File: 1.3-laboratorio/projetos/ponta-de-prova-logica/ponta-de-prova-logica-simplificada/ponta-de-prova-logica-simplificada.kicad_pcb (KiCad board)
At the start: 2 copper layers, 36.8 x 63.5 mm, 21 parts, among them J1 Conn_01x02, J2 PONTA DE PROVA, U1 LM339

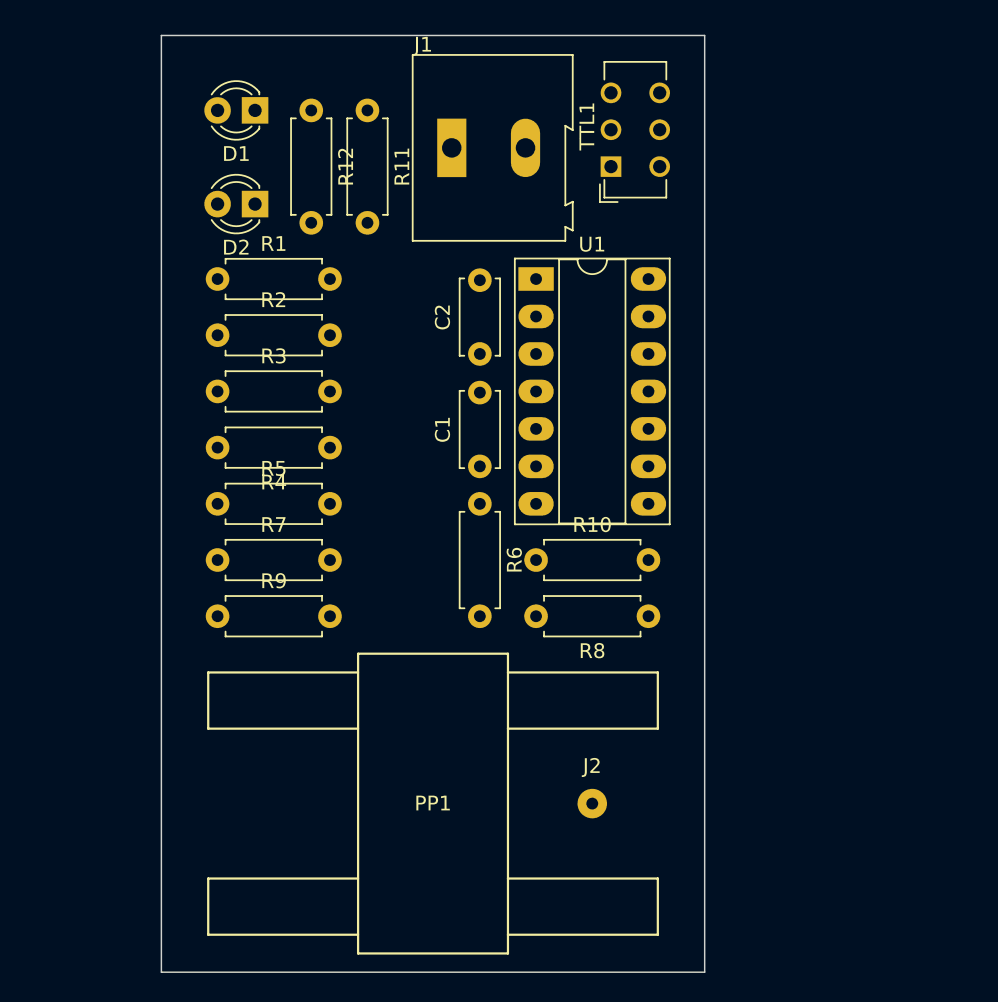
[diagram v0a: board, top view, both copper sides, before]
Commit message: Leiaute da PCB em andamento.
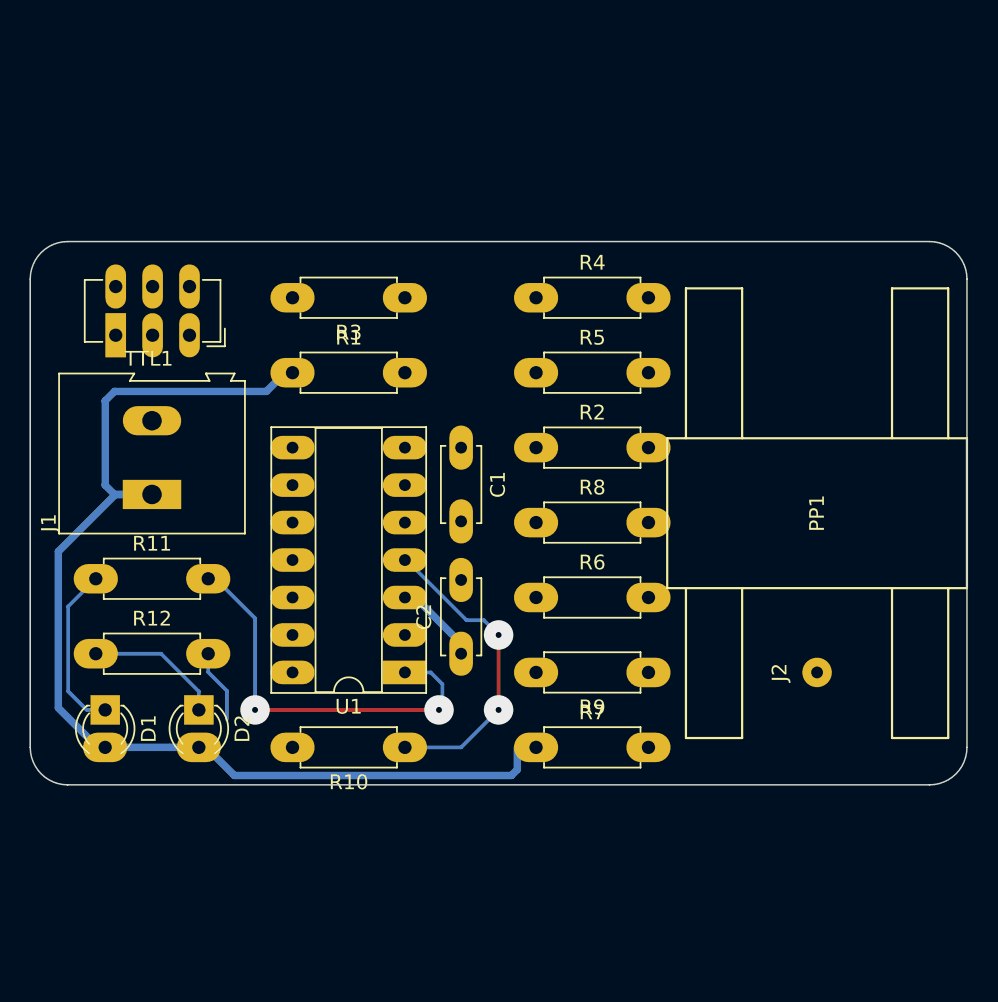
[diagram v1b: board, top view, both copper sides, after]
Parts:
- moved D1 41.9 mm to (134.6, 114.3), turned to 270 degrees
- moved R12 39.6 mm to (134.0, 110.5), turned to 0 degrees
- moved R11 36.7 mm to (134.0, 105.4), turned to 0 degrees
- moved D2 34.5 mm to (141.0, 114.3), turned to 270 degrees
- moved J1 31.1 mm to (137.8, 99.7), turned to 90 degrees
- moved TTL1 30.8 mm to (140.3, 88.9), turned to 180 degrees
- moved R9 29.5 mm to (171.4, 111.8), turned to 180 degrees
- moved U1 28.1 mm to (154.9, 111.8), turned to 180 degrees
- moved R7 25.0 mm to (163.8, 116.8)
- moved R5 23.3 mm to (163.8, 91.4)
- moved R2 22.9 mm to (163.8, 96.5)
- moved PP1 21.4 mm to (172.7, 106.0), turned to 90 degrees
- moved C2 20.4 mm to (158.8, 110.5)
- moved J2 17.6 mm to (182.9, 111.8), turned to 90 degrees
- moved R4 17.3 mm to (163.8, 86.4), turned to 0 degrees
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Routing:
- net VCC: track 0.00 -> 81.7 mm
- net Net-(R11-Pad2): track 0.00 -> 29.0 mm, vias 0 -> 2
- net Net-(R10-Pad1): track 0.00 -> 20.9 mm, vias 0 -> 2
- net Net-(D1-Pad1): track 0.00 -> 11.4 mm
- net Net-(D2-Pad1): track 0.00 -> 9.30 mm
- net Net-(R12-Pad2): track 0.00 -> 4.97 mm
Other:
- board size 36.8 x 63.5 mm -> 63.5 x 36.8 mm
- net class Default: trace_width 0.5 -> 0.25
- net class Vcc added: clearance 0.25, trace_width 0.5, via_dia 2, via_drill 0.4
- rule trace_min: 0.5 -> 0.25
